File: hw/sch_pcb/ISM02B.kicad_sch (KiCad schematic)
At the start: 58 parts, among them J1 JUMP_3X2, J10 HEADER_2x01_PARALLEL, J11 HEADER_2x01_PARALLEL, J12 SMA, J13 U.FL, J14 SMA, J15 U.FL, J16 BMI-S-204-F, J2 SM07B-GHS-TB, J3 HEADER_2x01_PARALLEL, J4 HEADER_2x01_PARALLEL, J5 HEADER_2x01_PARALLEL, J6 HEADER_2x01_PARALLEL, J7 HEADER_2x01_PARALLEL, J8 HEADER_2x01_PARALLEL, J9 HEADER_2x01_PARALLEL, M1 HOLE, M2 HOLE, M3 HOLE, M4 HOLE, U1 SX1262, U2 MIC5504-3.3YM5, Y1 32MHz

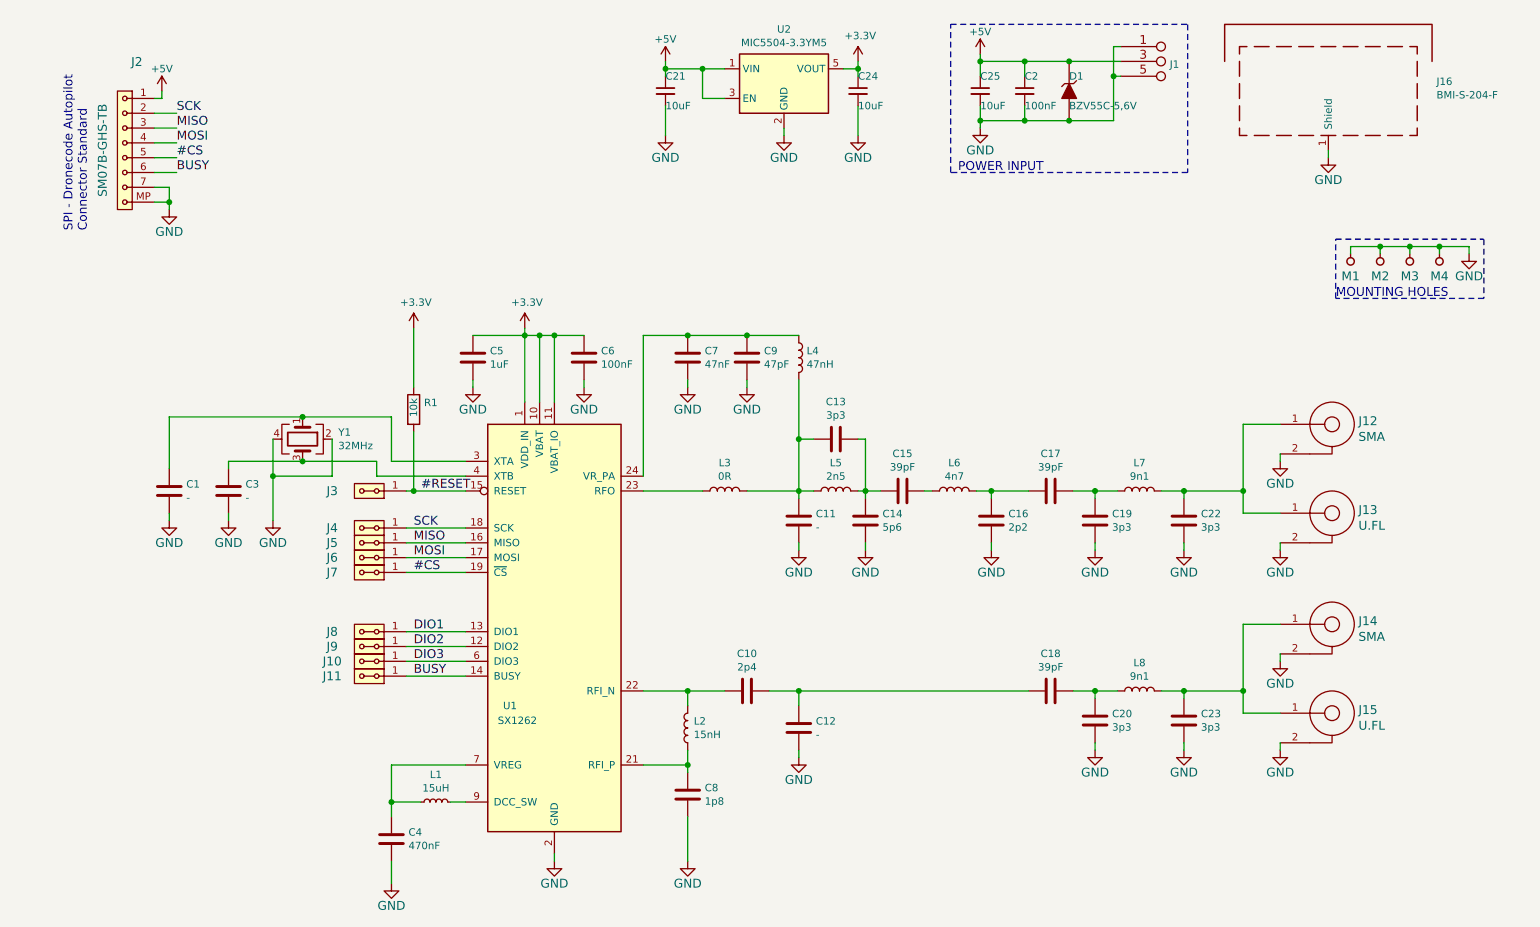
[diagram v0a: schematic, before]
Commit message: Edit
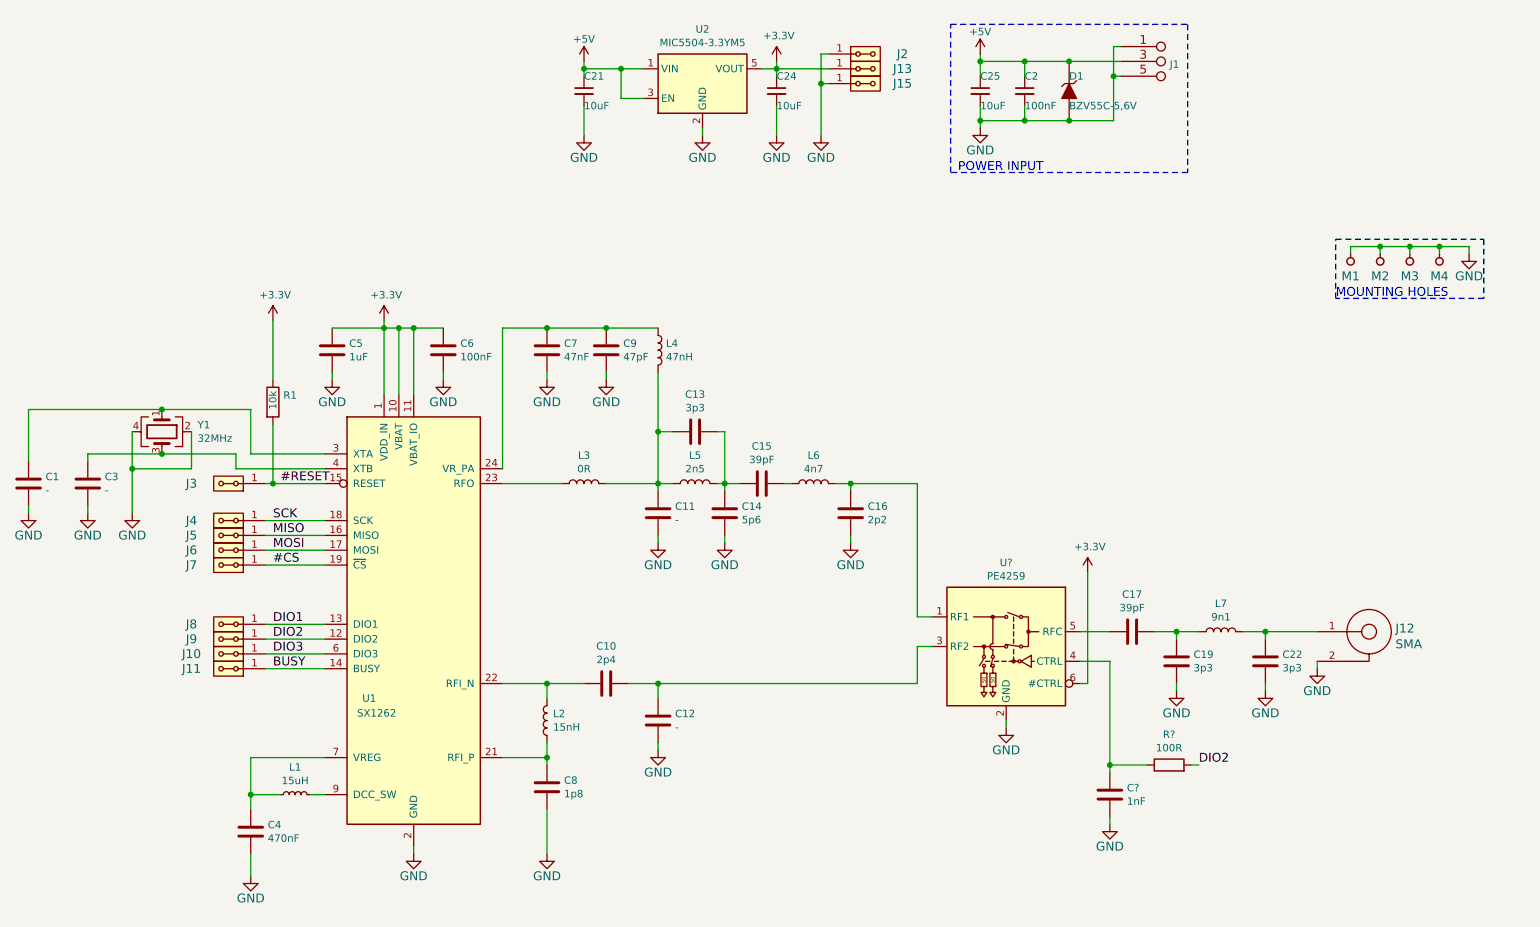
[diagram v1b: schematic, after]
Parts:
- removed C18: 39pF, Capacitor_SMD:C_0603_1608Metric_Pad1.05x0.95mm_HandSolder, symbol ISM02A-rescue:C-Device-ISM02A-rescue
- removed C20, C23: 3p3, Capacitor_SMD:C_0603_1608Metric_Pad1.05x0.95mm_HandSolder, symbol ISM02A-rescue:C-Device-ISM02A-rescue
- removed J13, J15: U.FL, Connector_Coaxial:U.FL_Hirose_U.FL-R-SMT-1_Vertical, symbol ISM02A-rescue:SMA-MLAB_CONNECTORS
- removed J14: SMA, Mlab_CON:SMA6251A13G50, symbol ISM02A-rescue:SMA-MLAB_CONNECTORS
- removed J16: BMI-S-204-F, MYLIB:BMI-S-204-F, symbol ISM02A-rescue:RF_Shield_Two_Pieces-device
- removed J2: SM07B-GHS-TB, Connector_JST:JST_GH_SM07B-GHS-TB_1x07-1MP_P1.25mm_Horizontal, symbol ISM02A-rescue:SM07B-GHS-TB-MLAB_CONNECTORS_JST-ISM02A-rescue
- removed L8: 9n1, Inductor_SMD:L_0402_1005Metric, symbol ISM02A-rescue:L-Device-ISM02A-rescue
- added C?: 1nF, symbol Device:C
- added J13, J15, J2: HEADER_2x01_PARALLEL, Mlab_Pin_Headers:Straight_2x01, symbol ISM02A-rescue:HEADER_2x01_PARALLEL-MLAB_HEADER
- added R?: 100R, symbol Device:R
- added U?: PE4259, Package_TO_SOT_SMD:SOT-363_SC-70-6, symbol MLAB_IO:PE4259
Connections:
- net +3V3: now also J13.1, J13.2, U?.6 (#CTRL)
- net DIO2: now also R?.2
- net GND: now also C?.2, J15.1, J15.2, J2.1, J2.2, U?.2 (GND)
- net at C16.1, L6.2: now also U?.1 (RF1); no longer C17.2
- net at C10.1, C12.1: now also U?.3 (RF2)
- new net: C17.2, U?.5 (RFC)
- new net: C?.1, R?.1, U?.4 (CTRL)
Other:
- note removed: "SPI - Dronecode Autopilot Connector Standard"
- moved on the sheet: C1, C10, C11, C12, C13, C14, C15, C16, C17, C19, C21, C22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
